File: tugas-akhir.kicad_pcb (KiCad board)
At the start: 2 copper layers, 120 x 100 mm, 32 parts, among them J1 Conn_01x02_Socket, J2 Conn_01x02_Pin (solenoid lini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, K1 Relay_SPDT, M1 Stepper_Motor_bipolar / Nema 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, M2 Stepper_Motor_bipolar / Nema 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, M3 Stepper_Motor_bipolar / Nema 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, Q1 2N3904, U1 ESP32-DEVKIT-V1, U2 DCDC_StepDown_LM2596, U3 TMC2208_SILENTSTEPSTICK, U4 TMC2208_SILENTSTEPSTICK, U5 TMC2208_SILENTSTEPSTICK

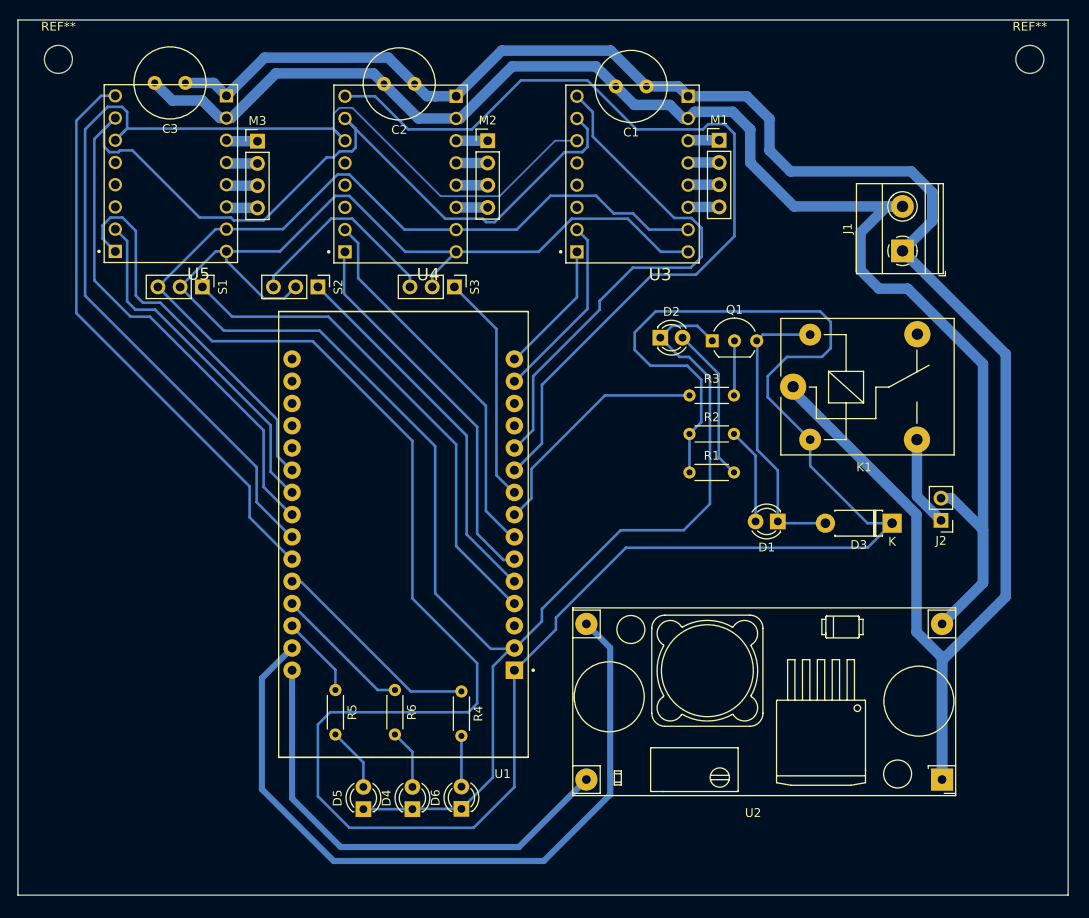
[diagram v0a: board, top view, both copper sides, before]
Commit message: finish pcb route
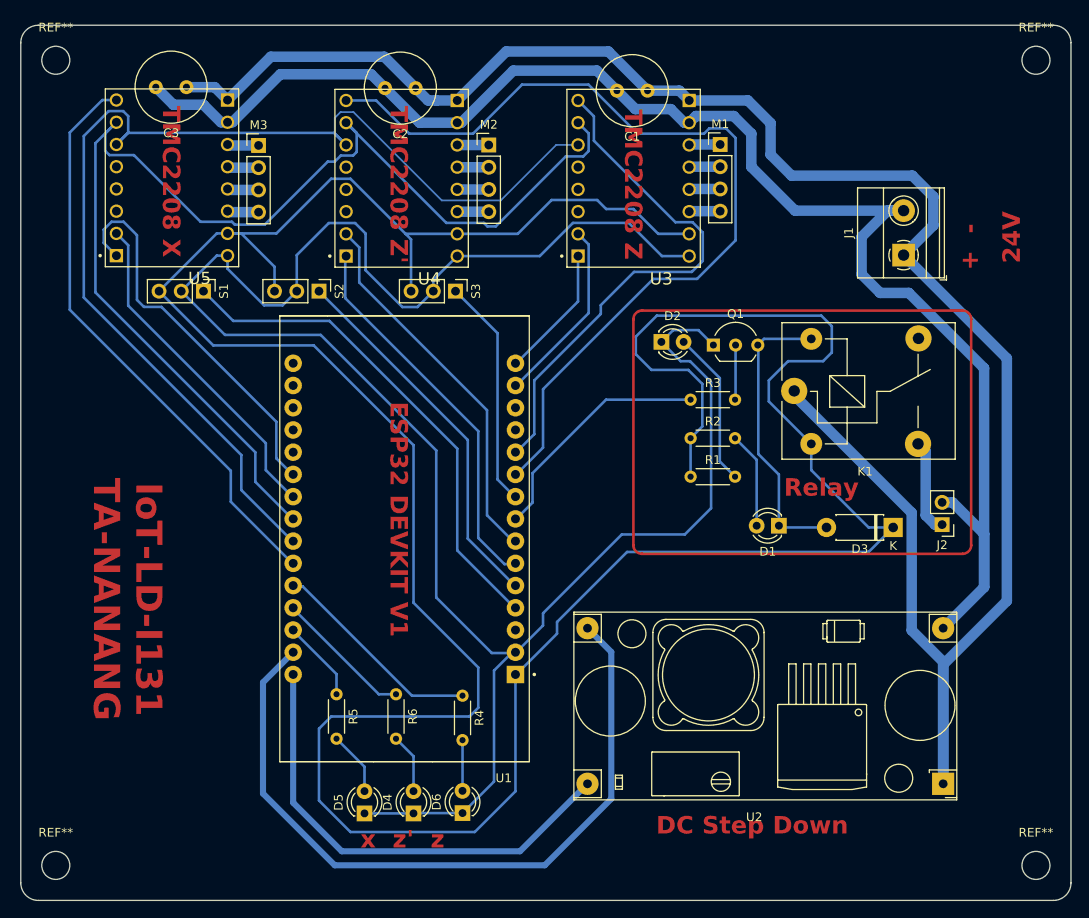
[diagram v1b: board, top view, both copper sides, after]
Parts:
- added REF**: MountingHole_3.2mm_M3_ISO14580, MountingHole:MountingHole_3.2mm_M3_ISO14580, F.Cu at (200.2, 138.6)
- added REF**: MountingHole_3.2mm_M3_ISO14580, MountingHole:MountingHole_3.2mm_M3_ISO14580, F.Cu at (88.2, 138.6)
- moved REF** 0.71 mm to (200.2, 46.6)
- moved D6 0.50 mm to (134.7, 132.6)
- moved U2 0.50 mm to (189.6, 129.3)
- moved C1 0.50 mm to (155.8, 50.1)
- moved C2 0.50 mm to (129.3, 49.8)
- moved C3 0.50 mm to (103.1, 49.7)
- moved D1 0.50 mm to (170.8, 99.8)
- moved D2 0.50 mm to (157.4, 78.8)
- moved D3 0.50 mm to (183.9, 100.0)
- moved J1 0.50 mm to (185.1, 68.9)
- moved J2 0.50 mm to (189.5, 99.7)
- moved K1 0.50 mm to (172.6, 84.4)
- moved M1 0.50 mm to (164.1, 56.2)
- moved M2 0.50 mm to (137.7, 56.3)
- moved M3 0.50 mm to (111.4, 56.3)
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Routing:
- net Net-(D3-K): track 364.1 -> 357.2 mm
- net Net-(D2-K): track 241.3 -> 238.7 mm
- net Net-(U1-D25): track 140.5 -> 139.0 mm
- net Net-(U1-D33): track 39.9 -> 38.5 mm
- net +24V: track 228.9 -> 229.7 mm
- net Net-(U1-D27): track 66.0 -> 66.8 mm
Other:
- outline, holes or cut-outs redrawn
- board text added: "+ -"
- board text added: "24V"
- board text added: "DC Step Down"
- board text added: "ESP32 DEVKIT V1"
- board text added: "IoT-LD-I131 TA-NANANG"
- board text added: "Relay"
- board text added: "TMC2208 X"
- board text added: "TMC2208 Z"
- board text added: "TMC2208 Z'"
- board text added: "x z' z"
